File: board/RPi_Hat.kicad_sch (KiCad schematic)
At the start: 39 parts, among them J1 PiHat, SW1 Pushbutton, SW2 Pushbutton, SW3 Pushbutton, SW4 Pushbutton, SW5 Pushbutton, SW6 Pushbutton, SW7 Pushbutton, SW8 Pushbutton

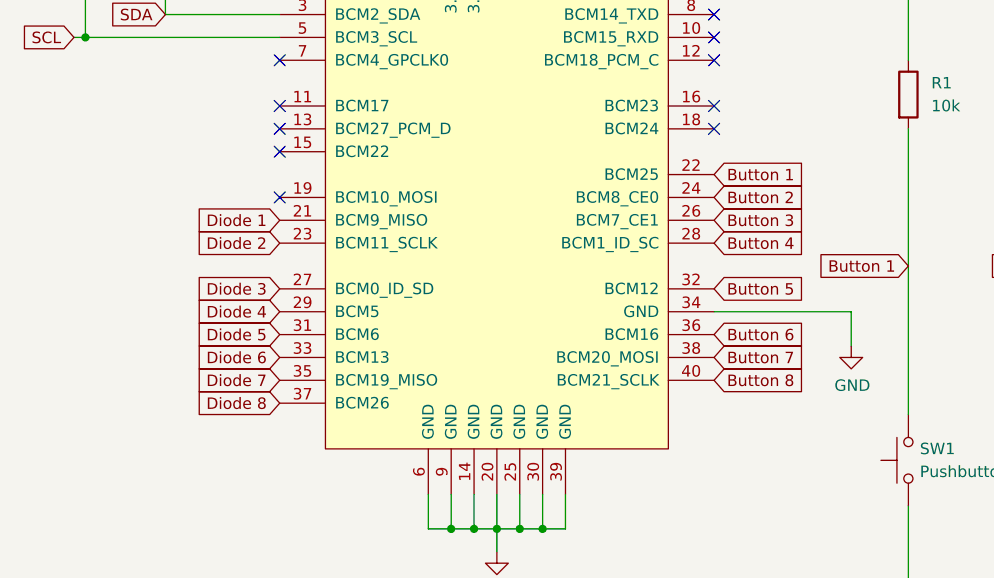
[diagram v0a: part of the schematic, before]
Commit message: pcb_completly_wired
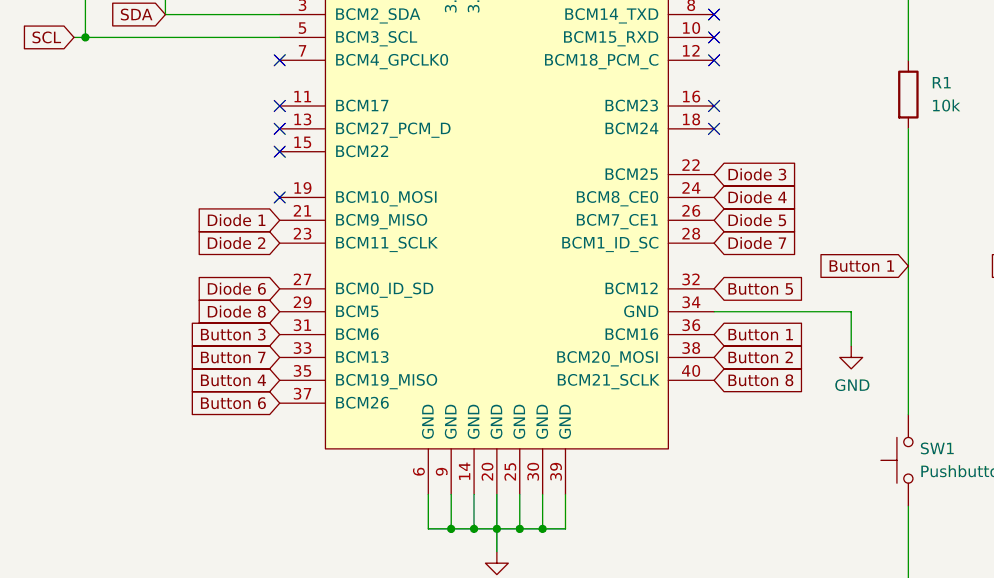
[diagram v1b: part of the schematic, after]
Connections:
- net Button 1: now also J1.36 (BCM16); no longer J1.22 (BCM25)
- net Button 2: now also J1.38 (BCM20_MOSI); no longer J1.24 (BCM8_CE0)
- net Button 3: now also J1.31 (BCM6); no longer J1.26 (BCM7_CE1)
- net Button 4: now also J1.35 (BCM19_MISO); no longer J1.28 (BCM1_ID_SC)
- net Button 6: now also J1.37 (BCM26); no longer J1.36 (BCM16)
- net Button 7: now also J1.33 (BCM13); no longer J1.38 (BCM20_MOSI)
- net Diode 3: now also J1.22 (BCM25); no longer J1.27 (BCM0_ID_SD)
- net Diode 4: now also J1.24 (BCM8_CE0); no longer J1.29 (BCM5)
- net Diode 5: now also J1.26 (BCM7_CE1); no longer J1.31 (BCM6)
- net Diode 6: now also J1.27 (BCM0_ID_SD); no longer J1.33 (BCM13)
- net Diode 7: now also J1.28 (BCM1_ID_SC); no longer J1.35 (BCM19_MISO)
- net Diode 8: now also J1.29 (BCM5); no longer J1.37 (BCM26)
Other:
- title: (none) -> Rasperry Pi Shield
